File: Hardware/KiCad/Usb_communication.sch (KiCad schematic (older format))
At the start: 22 parts, among them Q1 2N7002PW, U1 FT231XS

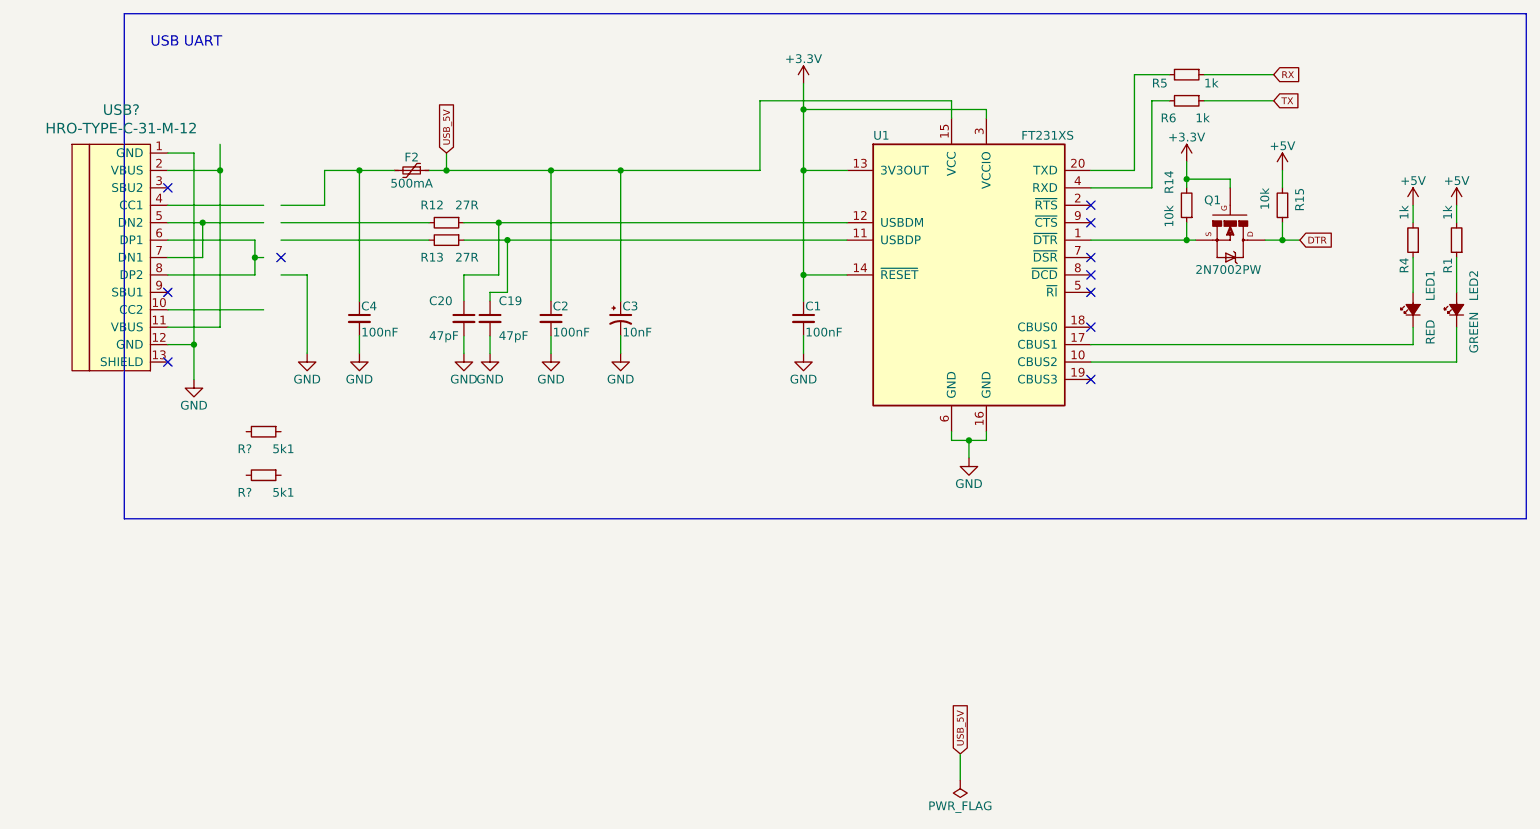
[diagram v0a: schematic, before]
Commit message: Conector y CH340C implementado
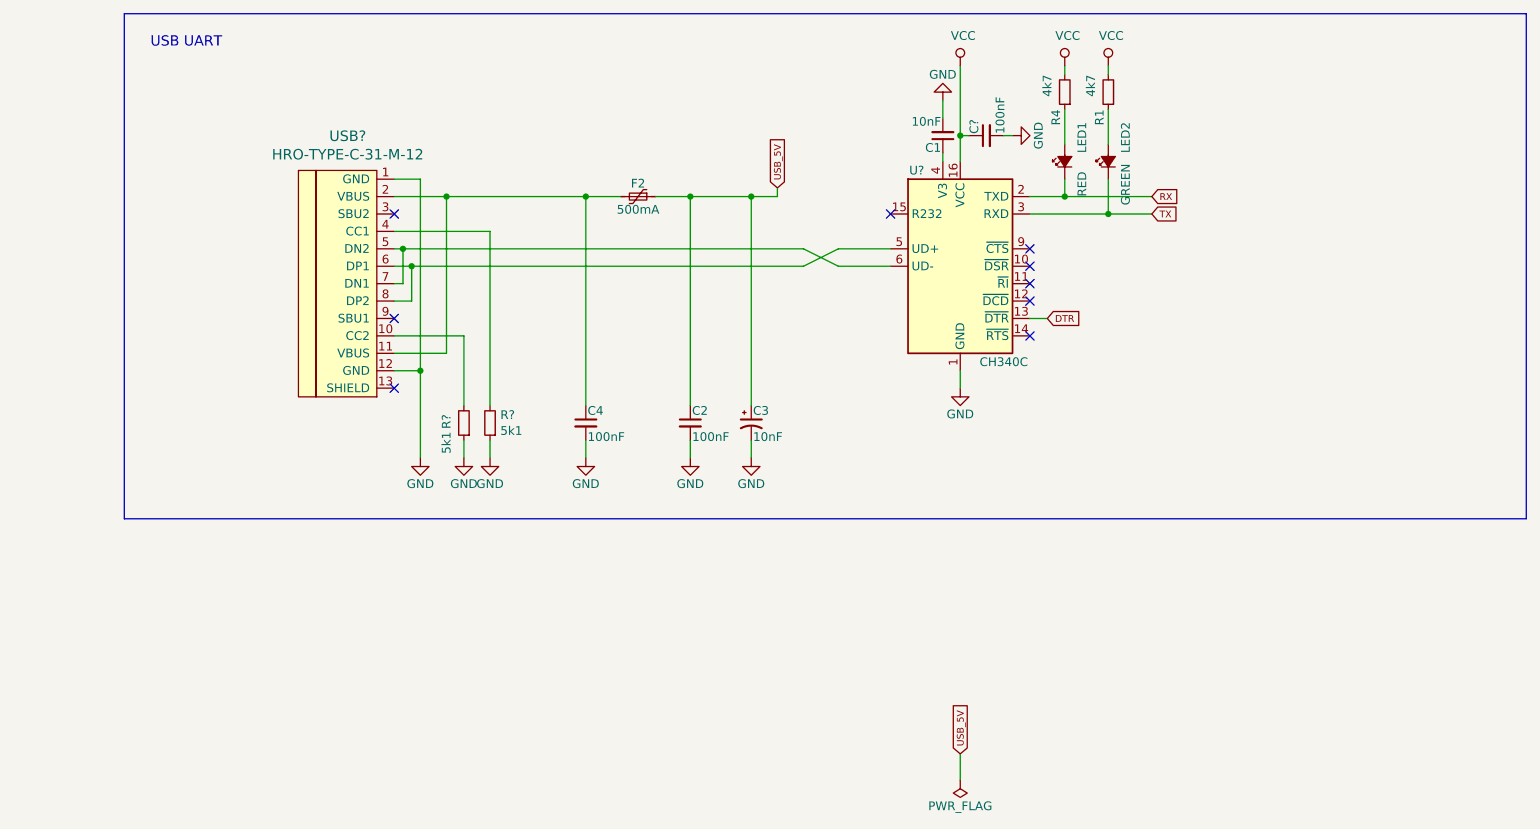
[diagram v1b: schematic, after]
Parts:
- removed C19, C20: 47pF, lib_sch:C_0805, symbol Grape:C_Small
- removed Q1: 2N7002PW, lib_sch:SOT-323_SC-70, symbol Grape:MOSFET-NCHANNEL2N7002PW
- removed R12, R13: 27R, lib_sch:R_0805, symbol Grape:R_Small
- removed R14, R15: 10k, lib_sch:R_0805, symbol Grape:R_Small
- removed R5, R6: 1k, lib_sch:R_0805, symbol Grape:R_Small
- removed R?: 5k1, lib_sch:R_0805, symbol Grape:R_Small
- removed U1: FT231XS, lib_sch:SSOP-20, symbol Grape:FT231XS
- added C?: 100nF, lib_sch:C_0805, symbol Grape:C_Small
- added R?: 5k1, lib_sch:R_0805, symbol Grape:R_Small
- added U?: CH340C, Package_SO:SOIC-16_3.9x9.9mm_P1.27mm, symbol Interface_USB:CH340C
- C1: value 100nF -> 10nF
- R1, R4: value 1k -> 4k7
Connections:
- net labels added: VCC
- net labels removed: +3.3V, +5V
- wire segments 95 -> 56
- no-connect marks 11 -> 9
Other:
- moved on the sheet: C1, C2, C3, C4, F2, LED1, LED2, R1, R4, R?, USB?
